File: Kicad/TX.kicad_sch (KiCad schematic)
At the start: 20 parts, among them J1 SI5351_breakout_board, Q1 Q_NMOS, U3 74AC00

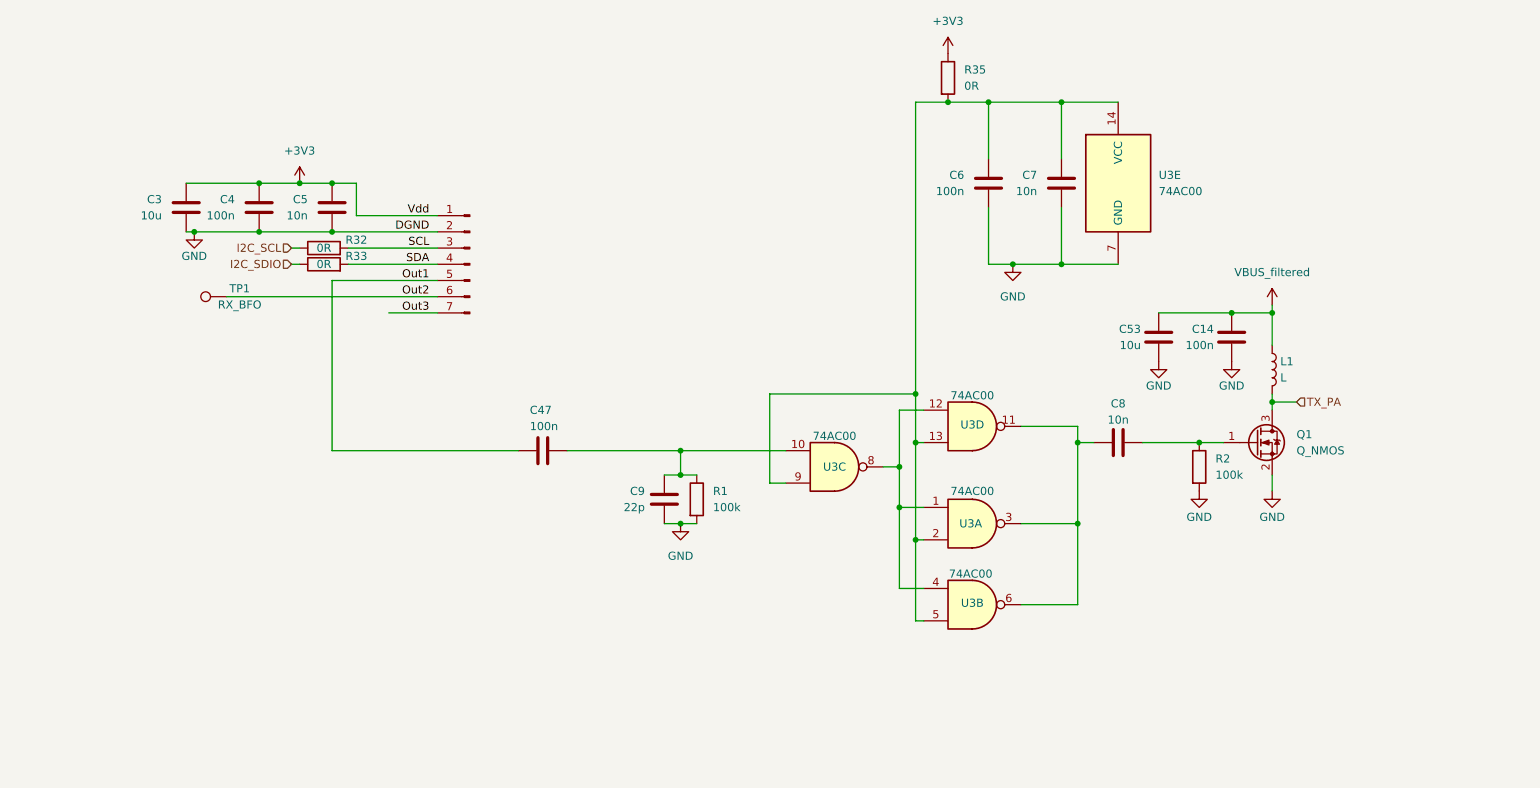
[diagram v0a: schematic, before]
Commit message: Add files via upload
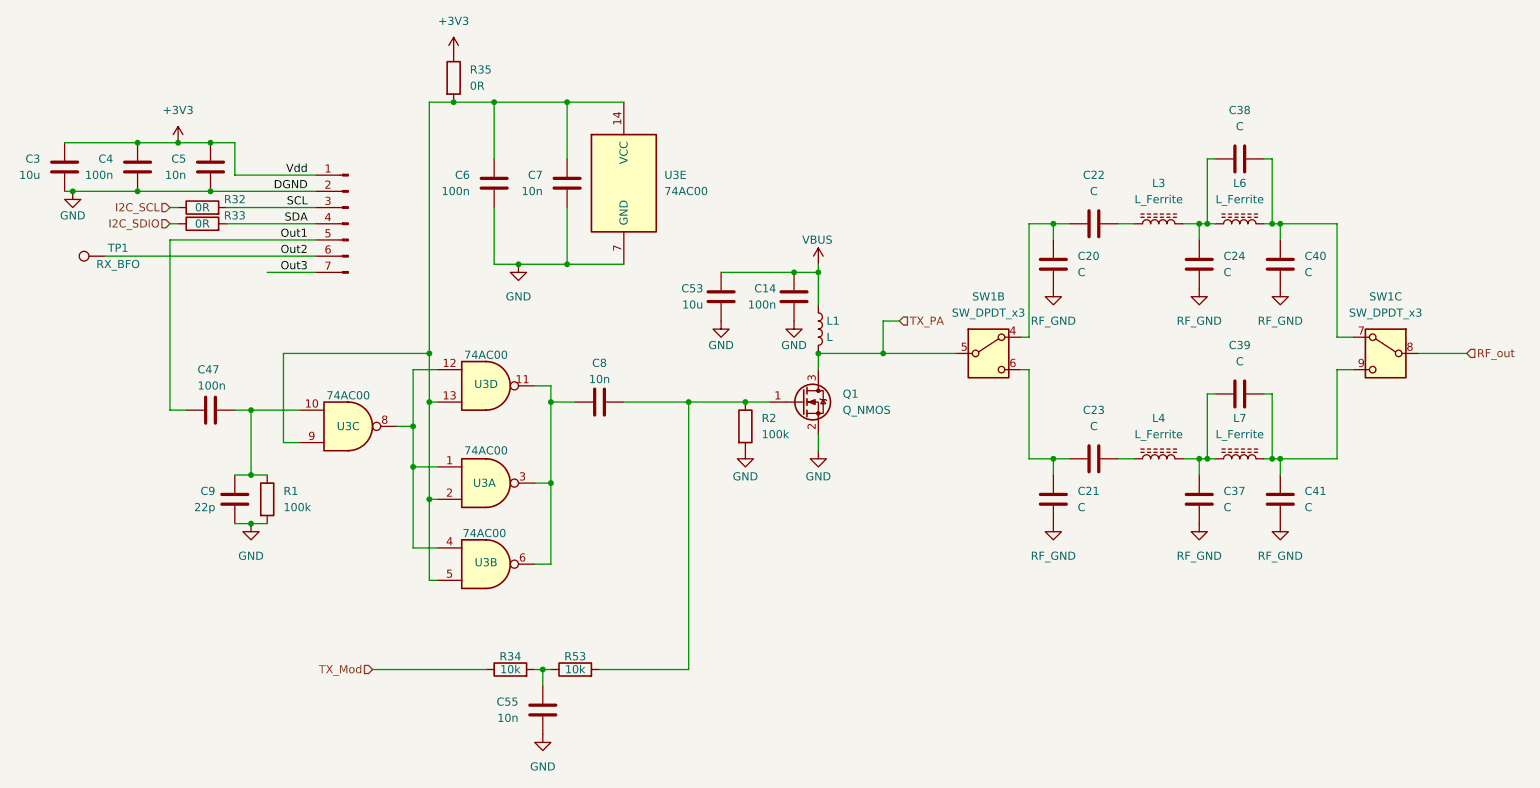
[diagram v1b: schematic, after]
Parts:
- added C20, C21, C22, C23, C24, C37, C38, C39, C40, C41: C, Capacitor_SMD:C_0603_1608Metric_Pad1.08x0.95mm_HandSolder, symbol Device:C
- added C55: 10n, Capacitor_SMD:C_0603_1608Metric_Pad1.08x0.95mm_HandSolder, symbol Device:C
- added L3, L4, L6, L7: L_Ferrite, Inductor_THT:L_Toroid_Vertical_L10.0mm_W5.0mm_P5.08mm, symbol Device:L_Ferrite
- added R34, R53: 10k, Resistor_SMD:R_0603_1608Metric, symbol Device:R
- added SW1: SW_DPDT_x3, summit_scourer:SW_GF-161-0005, symbol summit_scourer:SW_DPDT_x3
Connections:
- net GND: now also C55.2
- net TX_PA: now also SW1.5 (B)
- net at C8.2, Q1.1 (G), R2.1: now also R53.2
- net VBUS_filtered renamed VBUS
- new net: C55.1, R34.2, R53.1
- new net: C21.1, C23.1, SW1.6 (C)
- new net: C23.2, L4.1
- new net: C24.2, C38.1, L3.2, L6.1
- new net: C38.2, C40.1, L6.2, SW1.7 (A)
- new net: C20.1, C22.1, SW1.4 (A)
- new net: C22.2, L3.1
- new net: C39.2, C41.1, L7.2, SW1.9 (C)
- new net: C37.2, C39.1, L4.2, L7.1
- new net RF_GND: C20.2, C21.2, C24.1, C37.1, C40.2, C41.2
- new net RF_out: SW1.8 (B)
- new net TX_Mod: R34.1
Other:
- moved on the sheet: C14, C3, C4, C47, C5, C53, C6, C7, C8, C9, L1, Q1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
